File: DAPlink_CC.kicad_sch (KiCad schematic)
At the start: 20 parts

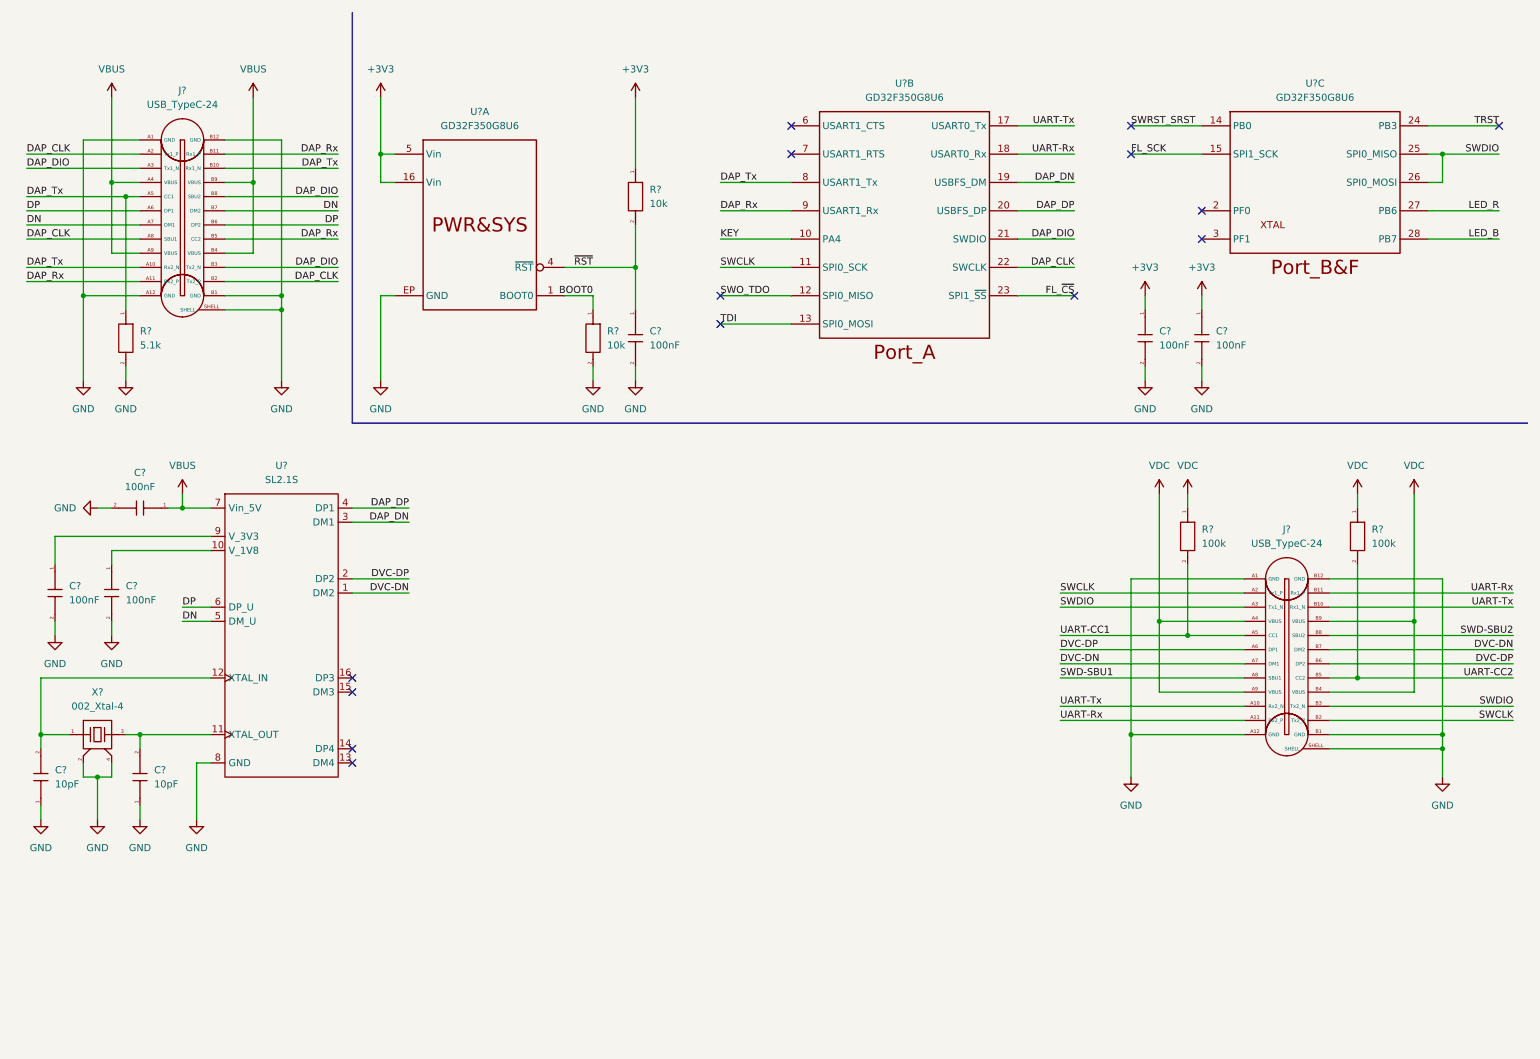
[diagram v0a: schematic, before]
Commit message: Update DAPlink_CC.kicad_sch
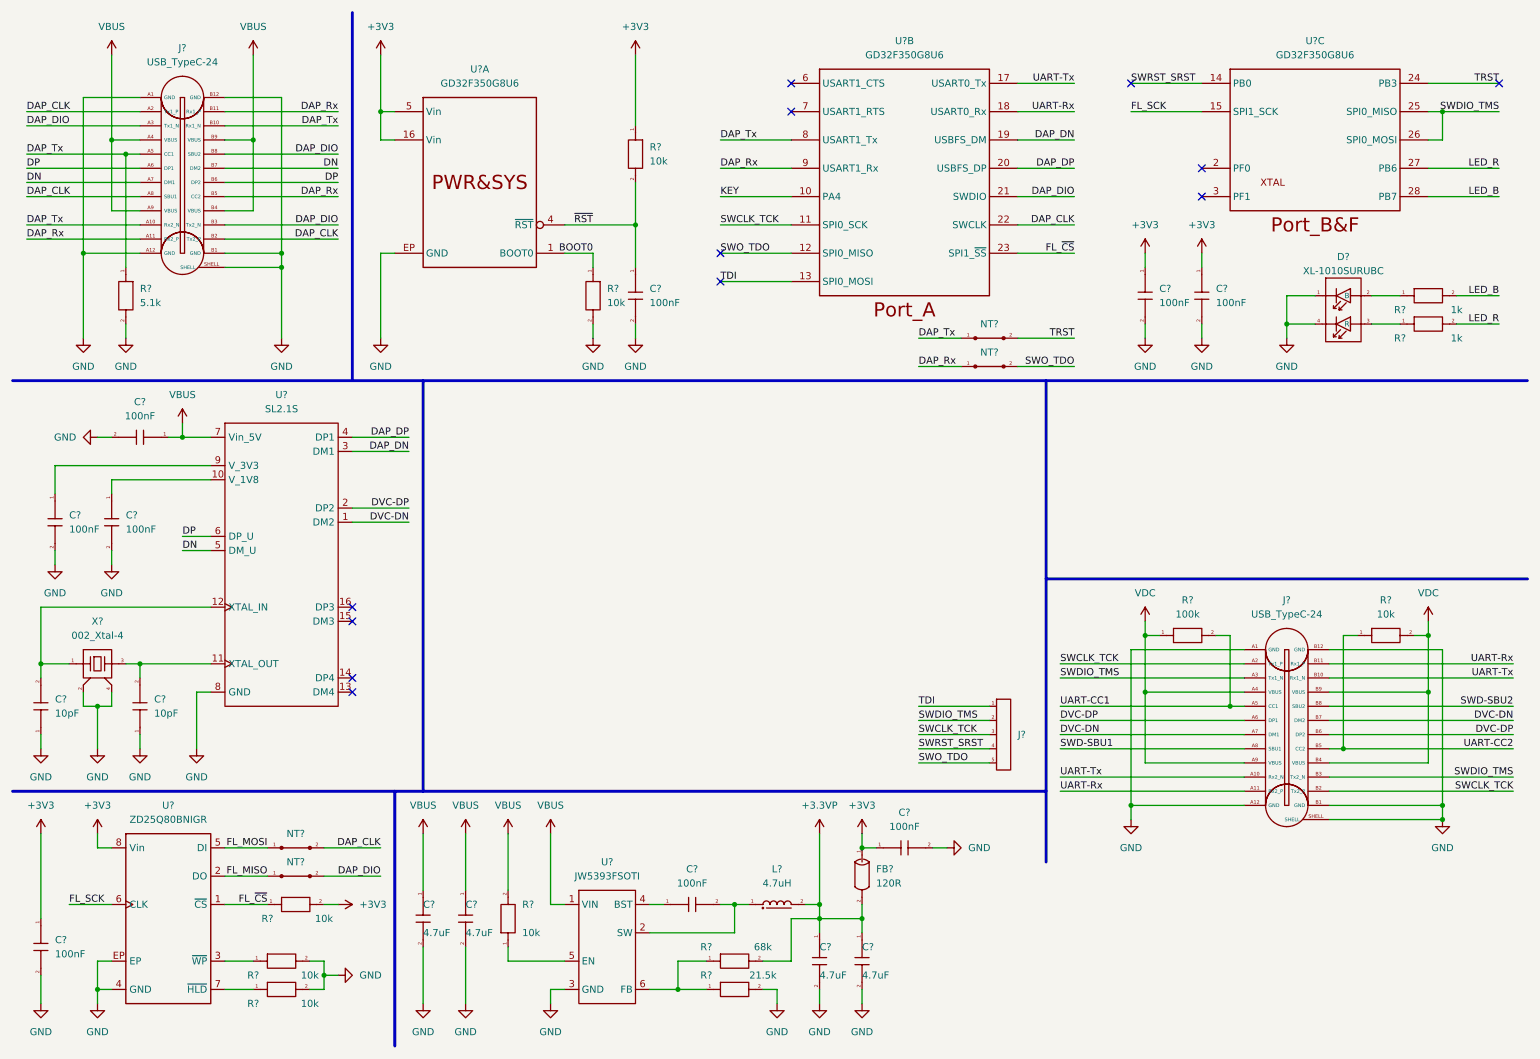
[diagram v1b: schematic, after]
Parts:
- removed C? (x5): 100nF, 001_GN_RCL_SMD:C0402(1005M), symbol 001_Basic_PassiveComponents:101_Capacitor
- removed C?: 10pF, 001_GN_RCL_SMD:C0402(1005M), symbol 001_Basic_PassiveComponents:101_Capacitor
- removed R? (x2): 100k, 001_GN_RCL_SMD:R0402(1005M), symbol 001_Basic_PassiveComponents:001_Resistor
- removed R?: 10k, 001_GN_RCL_SMD:R0402(1005M), symbol 001_Basic_PassiveComponents:001_Resistor
- added C?: 10pF, 001_GN_RCL_SMD:C0201(0603M), symbol 001_Basic_PassiveComponents:101_Capacitor
- added C? (x8): 100nF, 001_GN_RCL_SMD:C0201(0603M), symbol 001_Basic_PassiveComponents:101_Capacitor
- added C? (x4): 4.7uF, 001_GN_RCL_SMD:C0402(1005M), symbol 001_Basic_PassiveComponents:101_Capacitor
- added D?: XL-1010SURUBC, 003_GN_SMALL-SEMI_SMD:LED-4_1010, symbol 004_Basic_Co-PackagedSemiconductor:XL-1010SURUBC
- added FB?: 120R, 001_GN_RCL_SMD:L0603(1608M), symbol 001_Basic_PassiveComponents:301_FerriteBead
- added J?: Conn_01x05, symbol 302_Link_W2B-Connector:Conn_01x05
- added L?: 4.7uH, 008_GN_POWER-CHOKE_SMD:MC-0530, symbol 001_Basic_PassiveComponents:202_PowerChoke
- added NT? (x4): NetCNVT-2, symbol 300_Link_NetCNVT:NetCNVT-2
- added R?: 68k, 001_GN_RCL_SMD:R0201(0603M), symbol 001_Basic_PassiveComponents:001_Resistor
- added R? (x6): 10k, 001_GN_RCL_SMD:R0201(0603M), symbol 001_Basic_PassiveComponents:001_Resistor
- added R? (x2): 1k, 001_GN_RCL_SMD:R0201(0603M), symbol 001_Basic_PassiveComponents:001_Resistor
- added R?: 21.5k, 001_GN_RCL_SMD:R0201(0603M), symbol 001_Basic_PassiveComponents:001_Resistor
- added R?: 100k, 001_GN_RCL_SMD:R0201(0603M), symbol 001_Basic_PassiveComponents:001_Resistor
- added U?: JW5393FSOTI, 003_GN_SMALL-SEMI_SMD:SOT-563, symbol 204_Power_SMPS-Convertor:JW5393FSOTI
- added U?: ZD25Q80BNIGR, 003_GN_SMALL-SEMI_SMD:DFN-8_1515, symbol 108_IntegratedCircuit_Storage:ZD25Q80BNIGR
- C? (x2): footprint 001_GN_RCL_SMD:C0402(1005M) -> 001_GN_RCL_SMD:C0201(0603M)
- R? (x2): footprint 001_GN_RCL_SMD:R0402(1005M) -> 001_GN_RCL_SMD:R0201(0603M)
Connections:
- net +3V3: now also C?.1, C?.1, C?.1, C?.1, FB?.1, R?.2, U?.8 (Vin)
- net BOOT0: now also R?.1
- net DAP_CLK: now also NT?.2
- net DAP_DIO: now also NT?.2
- net DAP_Rx: now also NT?.1
- net DAP_Tx: now also NT?.1
- net FL_SCK: now also U?.6 (CLK)
- net FL_~{CS}: now also R?.1, U?.1 (~{CS})
- net GND: now also C?.1, C?.2, C?.2, C?.2, C?.2, C?.2, C?.2, C?.2, C?.2, C?.2, C?.2, C?.2, D?.1 (Cathode), D?.4 (Cathode), R?.2, R?.2, R?.2, R?.2, U?.3 (GND), U?.4 (GND), U?.EP
- net LED_B: now also R?.2
- net LED_R: now also R?.2
- net SWO_TDO: now also J?.5, NT?.2
- net SWRST_SRST: now also J?.4
- net TDI: now also J?.1
- net TRST: now also NT?.2
- net UART-CC1: now also R?.2
- net UART-CC2: now also R?.1
- net VBUS: now also C?.1, C?.1, R?.2, U?.1 (VIN)
- net VDC: now also R?.1, R?.2
- net ~{RST}: now also C?.1
- net at U?.10 (V_1V8): now also C?.1
- net at U?.11 (XTAL_OUT), X?.3: now also C?.2
- net at U?.9 (V_3V3): now also C?.1
- net SWCLK renamed SWCLK_TCK
- net SWCLK_TCK: now also J?.3
- net SWDIO renamed SWDIO_TMS
- net SWDIO_TMS: now also J?.2
- new net: R?.1, R?.1, U?.6 (FB)
- new net: R?.1, U?.7 (~{HLD})
- new net: D?.2 (Anode), R?.1
- new net: D?.3 (Anode), R?.1
- new net: C?.2, L?.1, U?.2 (SW)
- new net: C?.1, U?.4 (BST)
- new net: R?.1, U?.5 (EN)
- new net: R?.1, U?.3 (~{WP})
- new net +3.3VP: C?.1, C?.1, FB?.2, L?.2, R?.2
- new net FL_MISO: NT?.1, U?.2 (DO)
- new net FL_MOSI: NT?.1, U?.5 (DI)
- no-connect marks 14 -> 12
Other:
- moved on the sheet: C?, J?, R?, U?, U?A, U?B, U?C, X?
